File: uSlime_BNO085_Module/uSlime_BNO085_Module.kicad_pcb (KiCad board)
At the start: 2 copper layers, 13 parts, among them J1 Conn_01x05

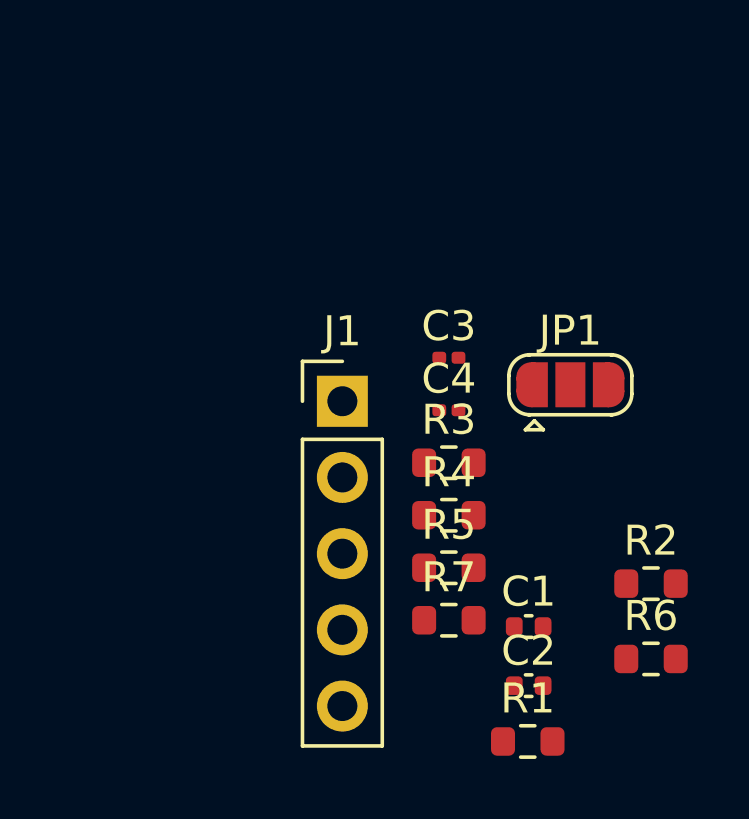
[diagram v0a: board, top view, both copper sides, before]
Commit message: update pcb design
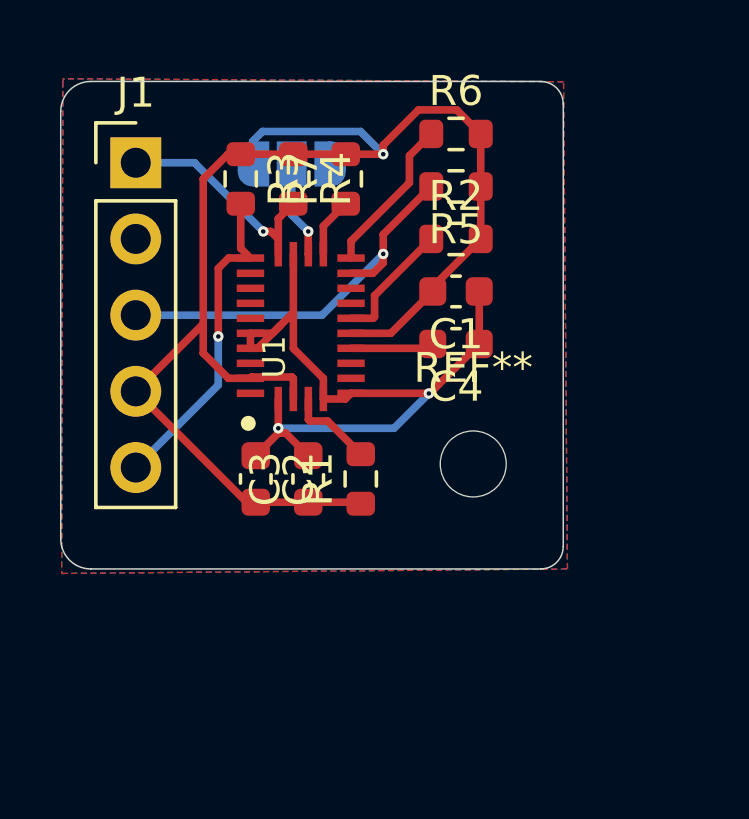
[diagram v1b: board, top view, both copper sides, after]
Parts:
- added REF**: MountingHole_2.2mm_M2, MountingHole:MountingHole_2.2mm_M2, F.Cu at (107.2, 107.1)
- added U1: BNO085, BNO_BreakOut:updatedBNO, F.Cu at (99.9, 103.9)
- C1, C2: footprint Capacitor_SMD:C_0402_1005Metric -> Capacitor_SMD:C_0603_1608Metric
- C3, C4: footprint Capacitor_SMD:C_0201_0603Metric -> Capacitor_SMD:C_0603_1608Metric
- JP1: moved to B.Cu
- moved R6 18.7 mm to (106.6, 96.1)
- moved R7 15.1 mm to (102.9, 97.6), turned to 90 degrees
- moved R2 13.2 mm to (106.6, 99.6)
- moved R5 12.7 mm to (106.6, 97.8), turned to 180 degrees
- moved R4 12.4 mm to (101.2, 97.6), turned to -90 degrees
- moved JP1 11.9 mm to (101.1, 97.1)
- moved R3 11.7 mm to (99.4, 97.6), turned to -90 degrees
- moved C1 11.4 mm to (106.6, 101.3), turned to 180 degrees
- moved C2 11.4 mm to (99.9, 107.6), turned to -90 degrees
- moved J1 10.5 mm to (95.9, 97.1)
- moved R1 10.4 mm to (103.4, 107.6), turned to 90 degrees
- moved C3 6.19 mm to (101.7, 107.6), turned to 90 degrees
- moved C4 2.22 mm to (106.6, 103.1), turned to 180 degrees
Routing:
- net +3.3V: track 0.00 -> 47.9 mm, vias 0 -> 1
- net GND: track 0.00 -> 25.4 mm, vias 0 -> 2
- net BNO_INT2: track 0.00 -> 14.0 mm, vias 0 -> 1
- net BNO_SDA: track 0.00 -> 10.9 mm, vias 0 -> 1
- net BNO_SCL: track 0.00 -> 7.69 mm, vias 0 -> 1
- net Net-(U1-ENV_SCL): track 0.00 -> 5.24 mm
- net Net-(U1-NRST): track 0.00 -> 4.18 mm
- net Net-(JP1-C): track 0.00 -> 3.24 mm, vias 0 -> 1
- net Net-(U1-BOOTN): track 0.00 -> 2.91 mm
- net Net-(U1-CAP): track 0.00 -> 2.78 mm
- net Net-(U1-ENV_SDA): track 0.00 -> 1.99 mm
- added copper zone on B.Cu, net GND
- added copper zone on F.Cu, net GND
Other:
- board outline added: 16.8 x 16.2 mm
- board text added: "4A"
- board text added: "4B"
